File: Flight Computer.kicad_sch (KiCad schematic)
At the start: 1 part, among them U6 STM32L476VETx

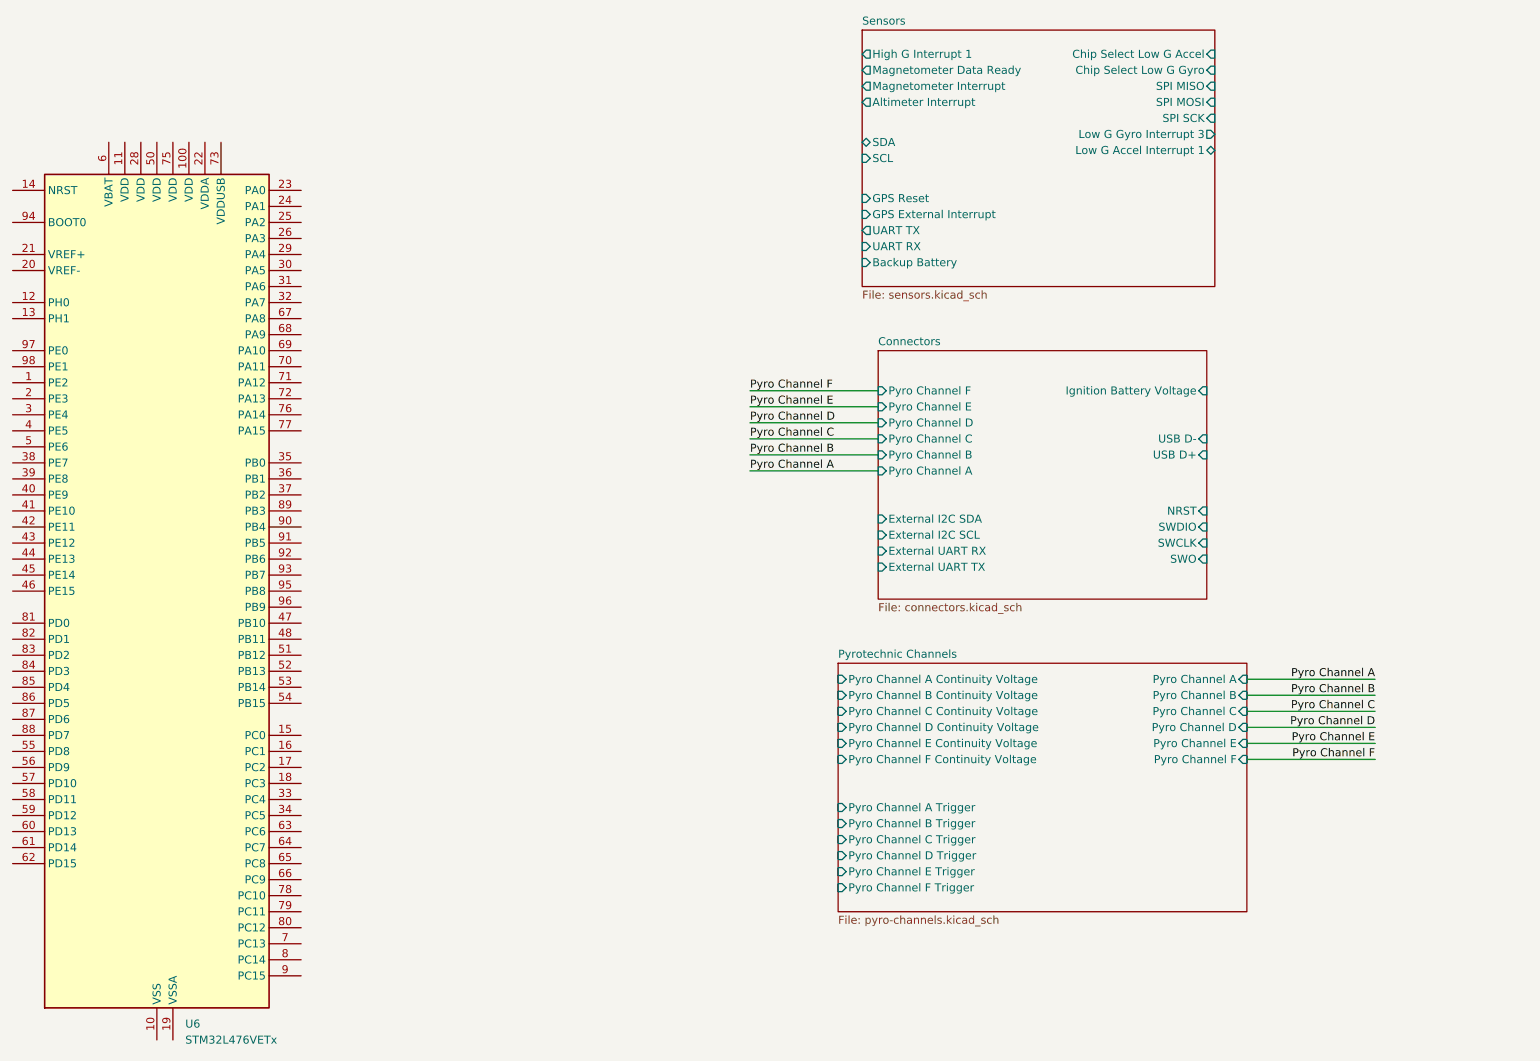
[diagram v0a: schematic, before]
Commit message: Began configuring STM32F476
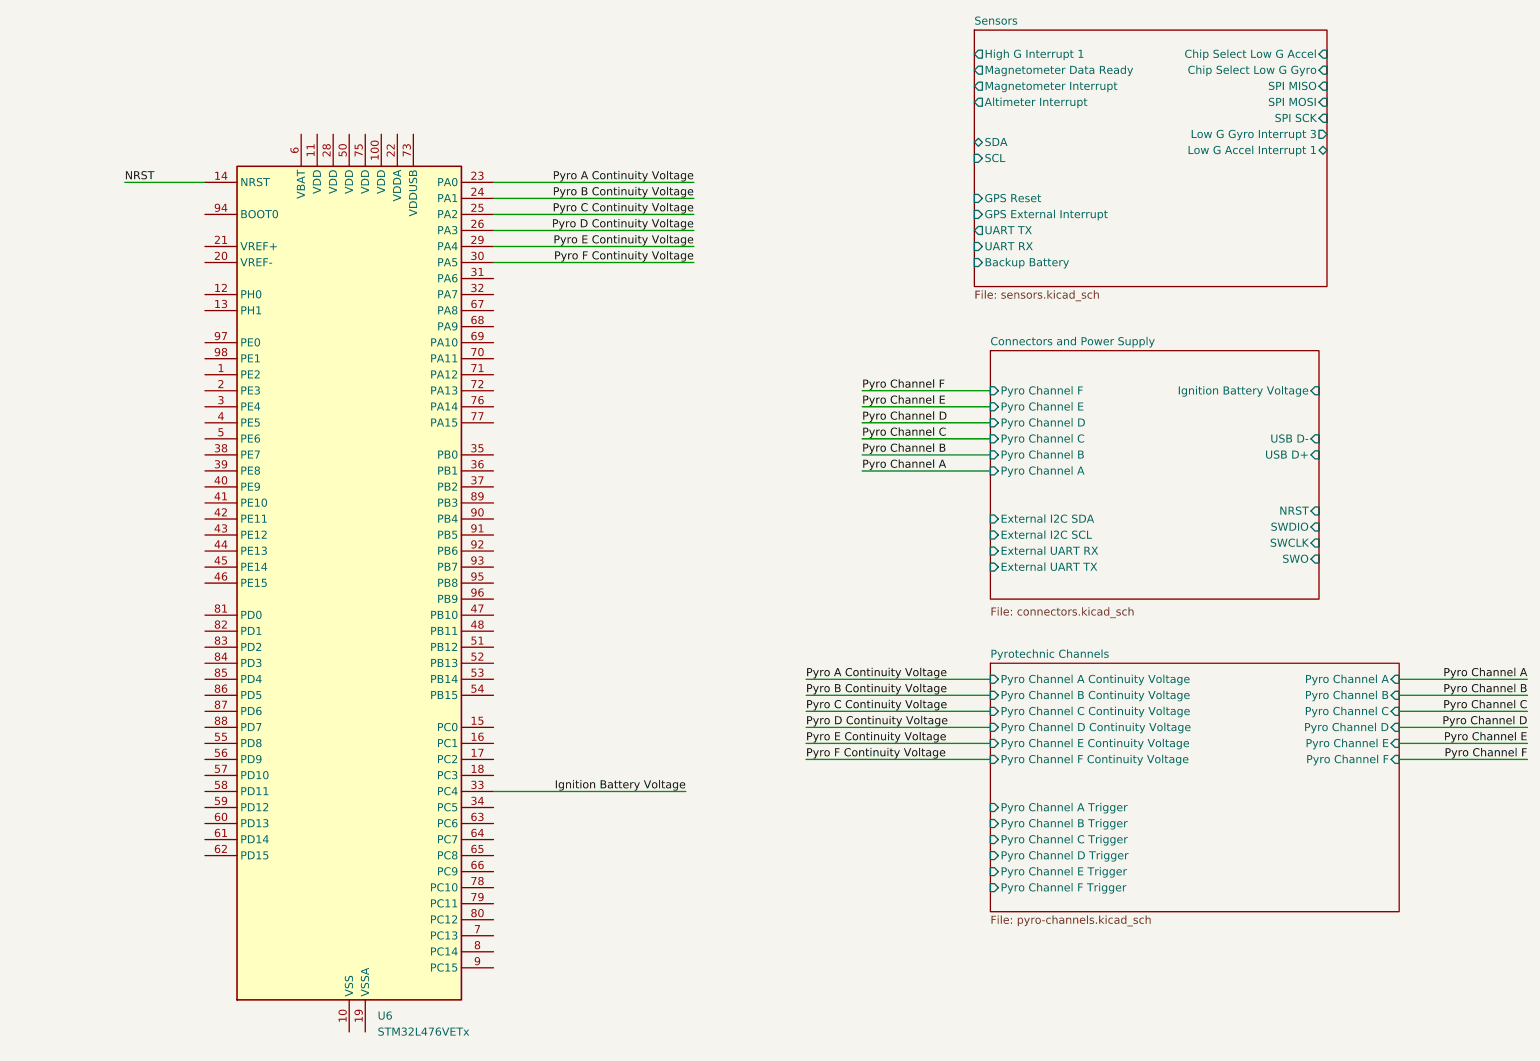
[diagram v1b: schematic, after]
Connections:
- net NRST: now reaches U6.14 (NRST)
- net Pyro A Continuity Voltage: now reaches U6.23 (PA0)
- net Pyro B Continuity Voltage: now reaches U6.24 (PA1)
- net Pyro C Continuity Voltage: now reaches U6.25 (PA2)
- net Pyro D Continuity Voltage: now reaches U6.26 (PA3)
- net Pyro E Continuity Voltage: now reaches U6.29 (PA4)
- net Pyro F Continuity Voltage: now reaches U6.30 (PA5)
- net Ignition Battery Voltage: now reaches U6.33 (PC4)
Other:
- sheet Connectors renamed Connectors and Power Supply
- moved on the sheet: U6
